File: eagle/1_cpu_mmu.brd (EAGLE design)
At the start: 28 parts, among them IC1 MT5C6408, IC10 74LS157N, IC11 74LS157N, IC12 74LS00N, IC13 74LS157N, IC14 74LS157N, IC15 74LS04N, IC19 74LS32N, IC2 MT5C6408, IC20 74LS02N, IC21 74LS374N, IC3 74LS27N, IC4 74LS20N, IC5 74LS08N, IC6 74LS245N, IC7 74LS245N, IC8 74LS32N, IC9 74LS157N

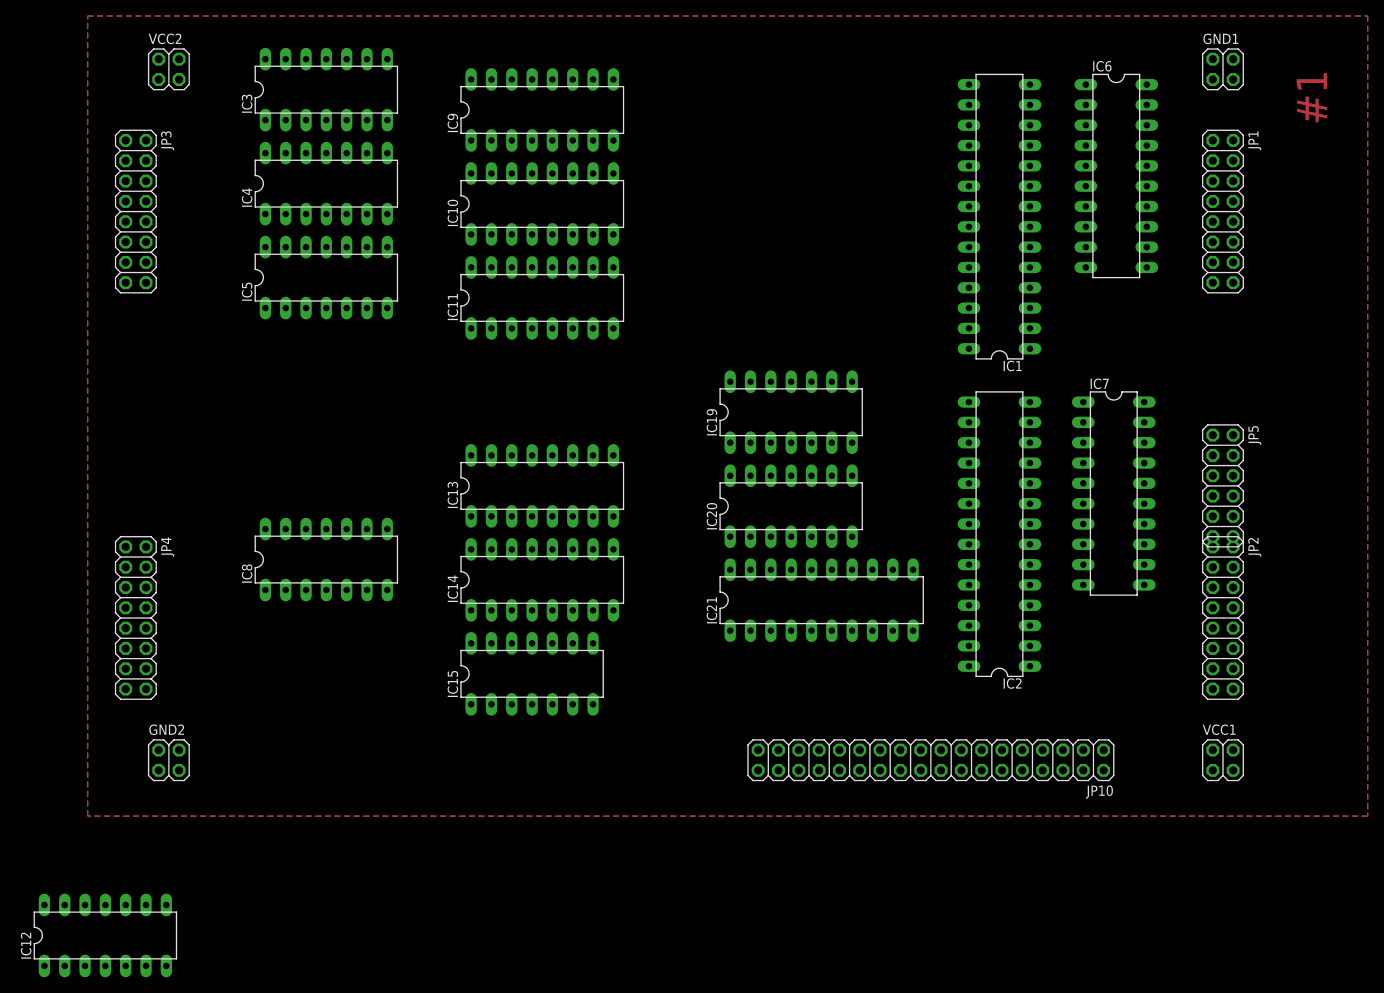
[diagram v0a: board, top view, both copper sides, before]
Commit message: MMU schematics completed
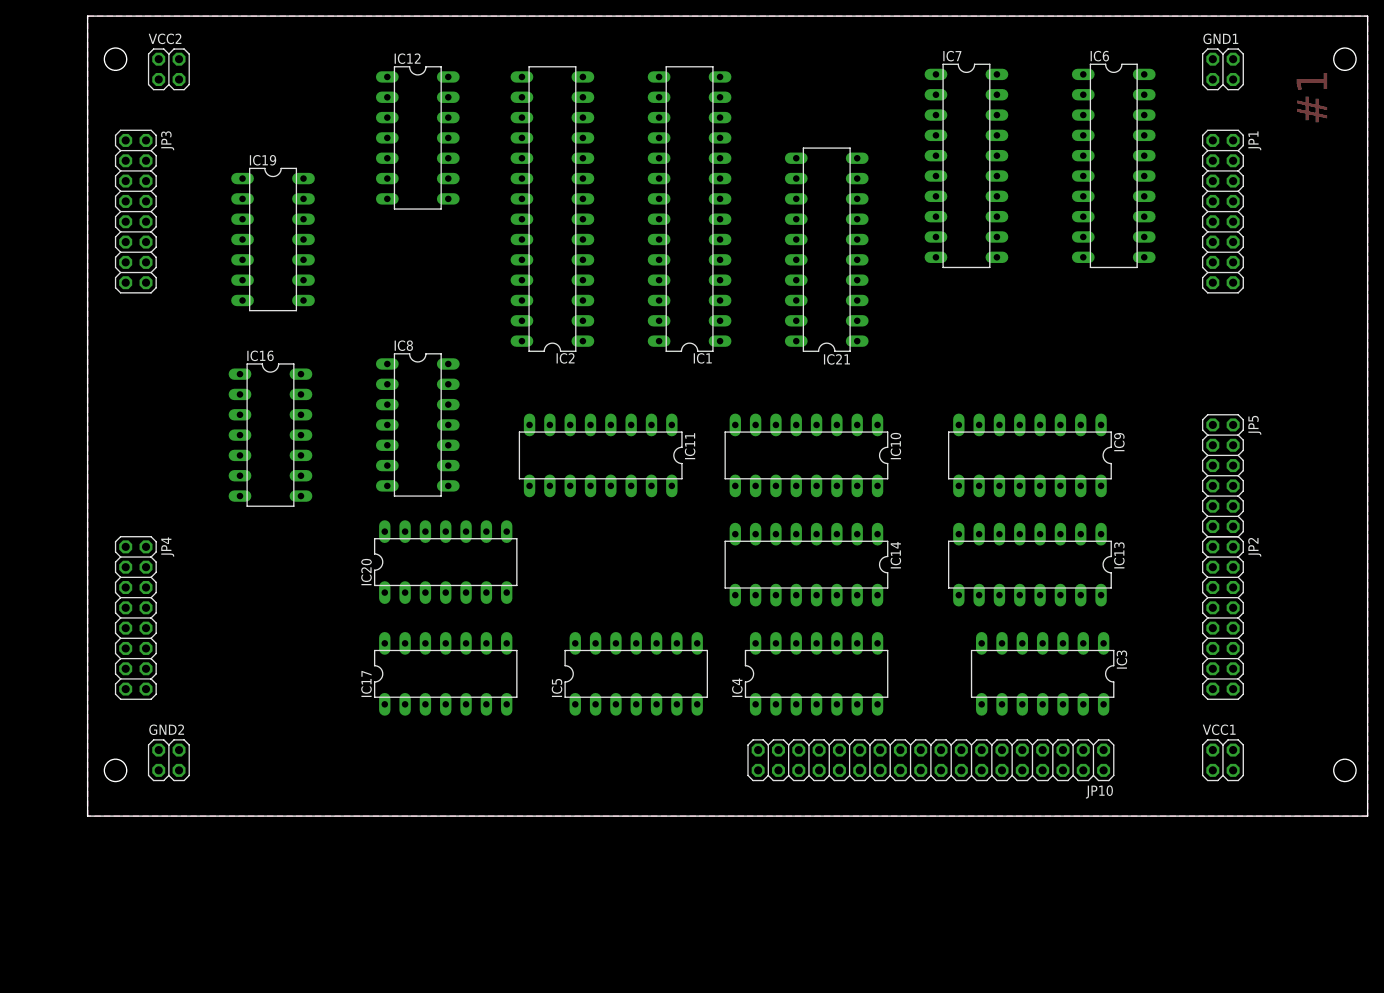
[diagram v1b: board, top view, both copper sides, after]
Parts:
- removed IC15: 74LS04N, 74xx-eu:DIL14
- added IC16: 74LS08N, 74xx-eu:DIL14
- added IC17: 74LS32N, 74xx-eu:DIL14
- moved IC3 115.5 mm to (119.4, 17.8), turned to 180 degrees
- moved IC12 107.1 mm to (41.3, 84.8), turned to 270 degrees
- moved IC4 86.7 mm to (91.1, 17.8)
- moved IC9 74.7 mm to (117.8, 45.1), turned to 180 degrees
- moved IC2 69.1 mm to (58.1, 75.9)
- moved IC19 68.3 mm to (23.2, 72.1), turned to 270 degrees
- moved IC5 62.9 mm to (68.6, 17.8)
- moved IC13 61.7 mm to (117.8, 31.4), turned to 180 degrees
- moved IC10 45.6 mm to (89.9, 45.1), turned to 180 degrees
- moved IC7 44.9 mm to (109.9, 81.3)
- moved IC21 43.8 mm to (92.4, 70.8), turned to 90 degrees
- moved IC20 43.7 mm to (44.8, 31.8)
- moved IC1 38.7 mm to (75.2, 75.9)
- moved IC14 33.1 mm to (89.9, 31.4), turned to 180 degrees
- moved IC11 21.0 mm to (64.1, 45.1), turned to 180 degrees
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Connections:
- removed net FIO: IC15.3, IC2.17, IC7.7
- removed net FPRESENT: IC2.19, IC7.9
- removed net FWRITABLE: IC2.18, IC7.8
- removed net N$18: IC11.11, IC15.4
- removed net N$19: IC12.2
- removed net N$31: IC12.1
- new net /FIO: IC11.11, IC2.17, IC7.7
- new net /FPRESENT: IC12.4, IC2.19, IC7.9
- new net /FWRITABLE: IC12.12, IC2.18, IC7.8
- new net N$33: IC12.5, IC20.1, IC5.4
- new net N$34: IC12.13, IC5.6
- net /ENMEM: now also IC17.2, IC5.5
- net /ENMEMX: now also IC17.3
- net /FP: now also IC17.10; no longer IC19.2
- net /LDMEM: now also IC17.5
- net /LDMEMX: now also IC17.6
- net /MEMOP: now also IC17.9; no longer IC19.1
- net /NP_FAULT: now also IC12.6, IC16.4
- net /WR_FAULT: now also IC12.11, IC16.5
- net ABUS0: now also IC12.2; no longer IC15.1
- net GND: now also IC16.7, IC17.7; no longer IC10.6, IC15.7
- net MEMSEG: now also IC10.6
- net N$20: now also IC17.8, IC20.2; no longer IC19.3, IC19.4
- net N$30: now also IC12.3; no longer IC15.2
- net N$32: now also IC17.1, IC17.4, IC20.3; no longer IC19.5
- net N$40: now also IC16.6; no longer IC12.3
- net VCC: now also IC16.14, IC17.14; no longer IC15.14
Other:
- board outline added: 160 x 100 mm
